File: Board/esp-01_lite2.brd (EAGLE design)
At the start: 17.4 x 49.5 mm, 21 parts, among them IC1 TINY13-20SU, K1 setup, K2 reset, X1 IN1, X2 IN2

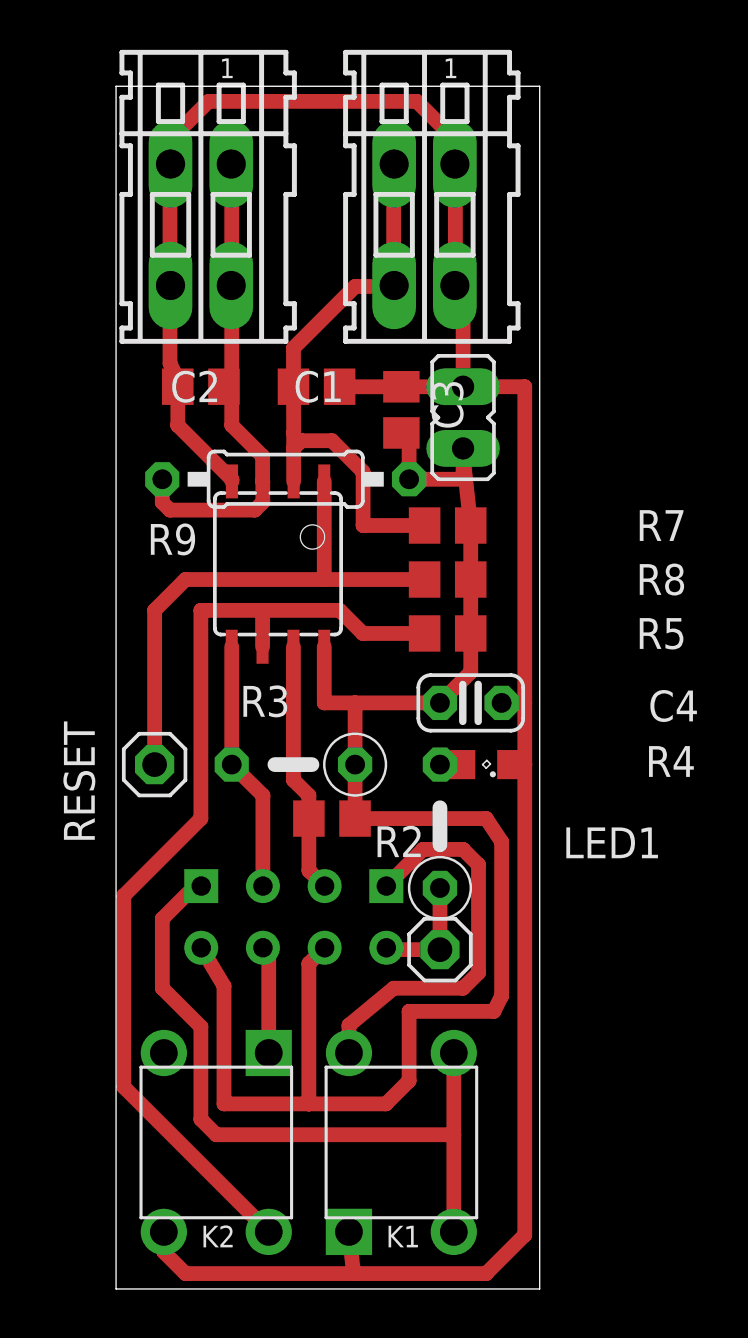
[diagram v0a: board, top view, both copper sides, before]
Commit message: scheme
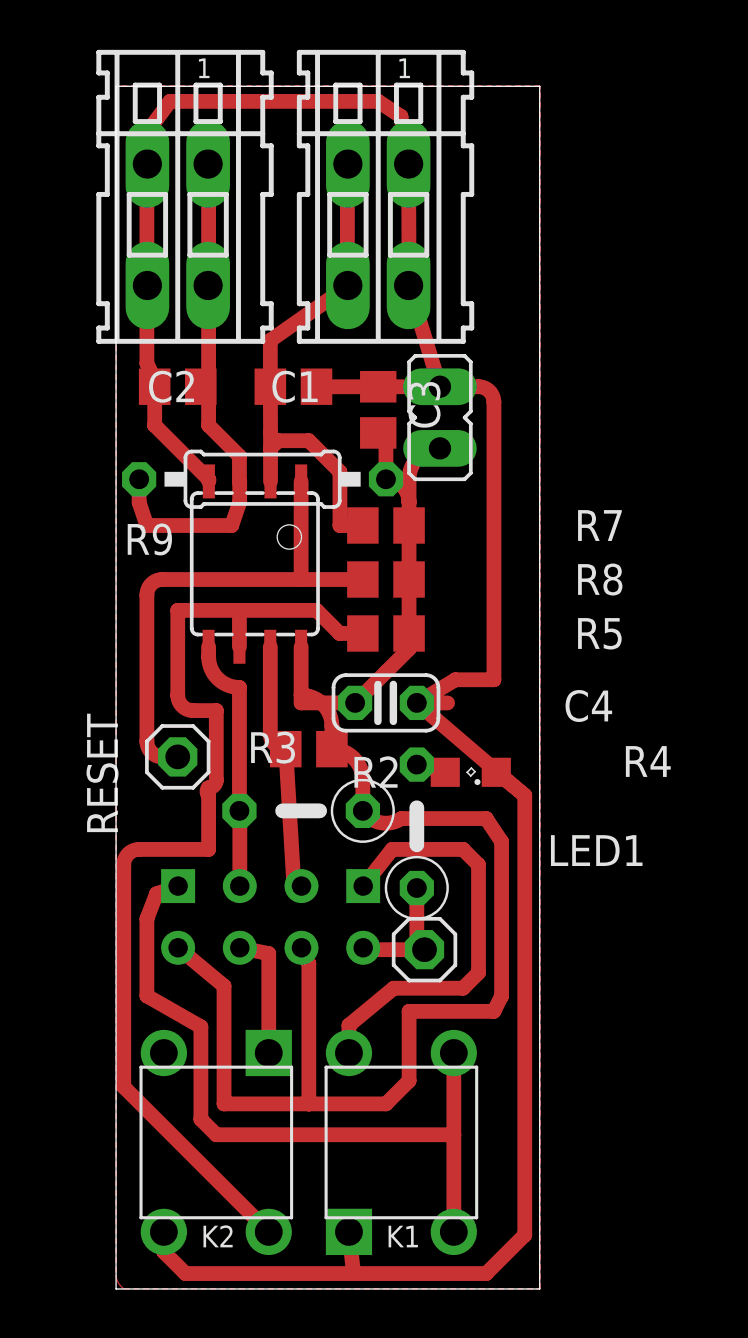
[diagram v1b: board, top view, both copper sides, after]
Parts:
- moved C4 3.49 mm to (11.1, 24.1)
- moved R2 3.01 mm to (7.94, 22.2)
- moved R5 2.54 mm to (11.1, 27.0)
- moved R7 2.54 mm to (11.1, 31.4)
- moved R8 2.54 mm to (11.1, 29.2)
- moved R3 1.93 mm to (7.62, 19.7)
- moved X1 1.90 mm to (10.8, 43.8)
- moved RESET 1.00 mm to (2.54, 21.9)
- moved C1 0.95 mm to (7.30, 37.1)
- moved C3 0.95 mm to (10.8, 36.2)
- moved IC1 0.95 mm to (5.71, 29.8)
- moved R4 0.95 mm to (12.4, 19.1)
- moved R9 0.95 mm to (6.03, 33.3)
- moved U$1 0.95 mm to (6.35, 22.2)
- moved C2 0.95 mm to (2.54, 37.1)
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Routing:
- net GND: track 102.2 -> 107.9 mm
- net +3V3: track 70.6 -> 67.4 mm
- net N$9: track 24.0 -> 21.4 mm
- net N$5: track 40.5 -> 42.0 mm
- net N$13: track 22.0 -> 20.8 mm
- net N$15: track 20.3 -> 21.4 mm
- net N$10: track 16.4 -> 17.5 mm
- net N$8: track 4.43 -> 5.31 mm
- net N$4: track 29.1 -> 29.6 mm
- added copper zone on layer 1, net GND
